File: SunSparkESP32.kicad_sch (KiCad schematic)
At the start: 50 parts, among them J1 Conn_01x02_Pin, J2 USB_C_Receptacle_USB2.0, J4 Conn_01x15_Pin, J5 Conn_01x03_Pin, J6 Conn_01x15_Pin, J7 Conn_01x01_Pin, Q1 IRLML6244TRPBF, Q2 IRLML6244TRPBF, SW1 SW_Push, SW2 SW_Push, U1 ADP5090ACP, U2 AMS1117-3.3, U3 ESP32-S2-MINI-1, U4 RFM96W-433S2

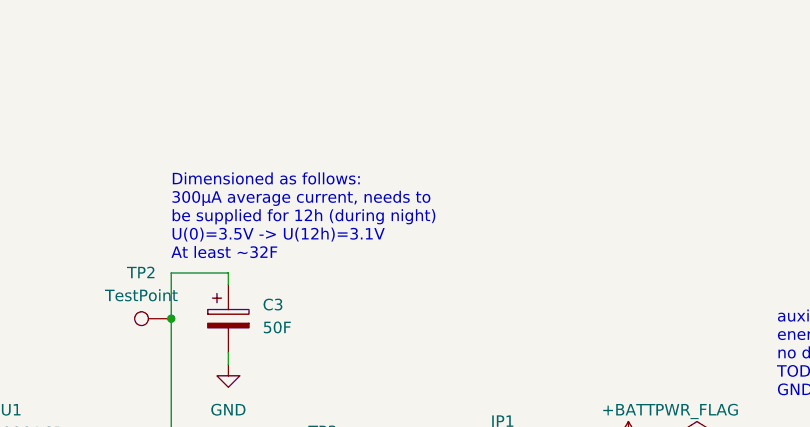
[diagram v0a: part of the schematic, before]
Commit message: Minor improvements on documentation
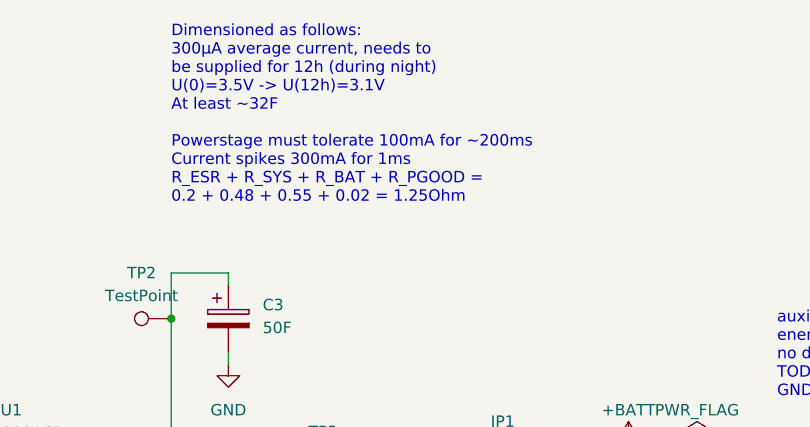
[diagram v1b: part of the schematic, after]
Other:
- note added: "Dimensioned as follows: 300µA average current, needs to be supplied for 12h (during night) U(0)=3.5V -> U(12h)=3.1V At least ~32F Powerstage must tolerate 100mA for ~200ms Current spikes 300mA for 1ms R_ESR + R_SYS + R_BAT + R_PGOOD = 0.2 + 0.48 + 0.55 + 0.02 = 1.25Ohm"
- note removed: "Dimensioned as follows: 300µA average current, needs to be supplied for 12h (during night) U(0)=3.5V -> U(12h)=3.1V At least ~32F"
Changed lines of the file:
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@@
     (effects (font (size 1.27 1.27)) (justify left bottom))
   )
-  (text "Dimensioned as follows:\n300µA average current, needs to\nbe supplied for 12h (during night)\nU(0)=3.5V -> U(12h)=3.1V\nAt least ~32F"
-    (at 106.68 52.07 0)
+  (text "Dimensioned as follows:\n300µA average current, needs to\nbe supplied for 12h (during night)\nU(0)=3.5V -> U(12h)=3.1V\nAt least ~32F\n\nPowerstage must tolerate 100mA for ~200ms\nCurrent spikes 300mA for 1ms\nR_ESR + R_SYS + R_BAT + R_PGOOD =\n0.2 + 0.48 + 0.55 + 0.02 = 1.25Ohm"
+    (at 106.68 45.72 0)
     (effects (font (size 1.27 1.27)) (justify left bottom))
   )
